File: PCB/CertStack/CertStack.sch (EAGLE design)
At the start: 46 parts, among them J1 MEM2075-00-140-01-A, Q1 SI2302, Q2 SI2302, Q3 SI2302, Q4 SI2302, Q5 MMBT2222A, T1 DMP3098L-7, U1 LT1374CS8-5PBF, U2 INVENSENSE_ICM-20608-GINVENSE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, U3 SST26VF064B-104V/MN

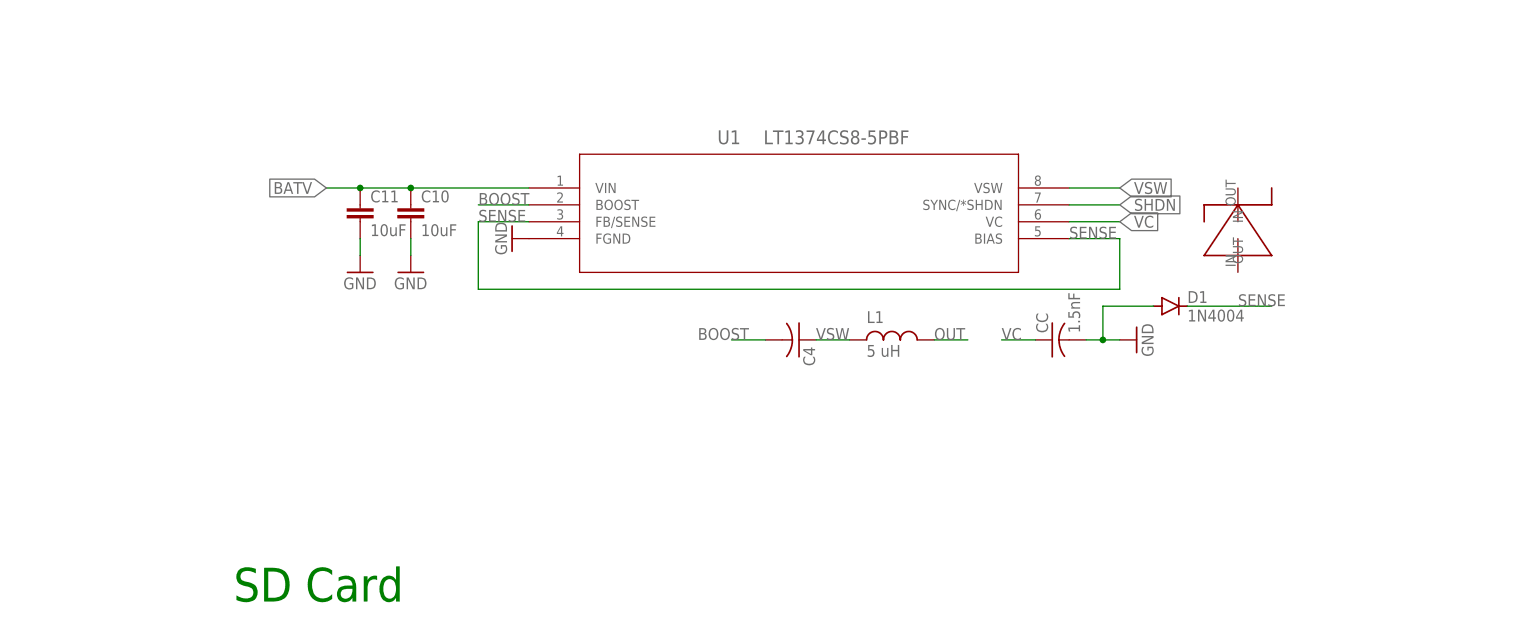
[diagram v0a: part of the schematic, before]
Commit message: PCB
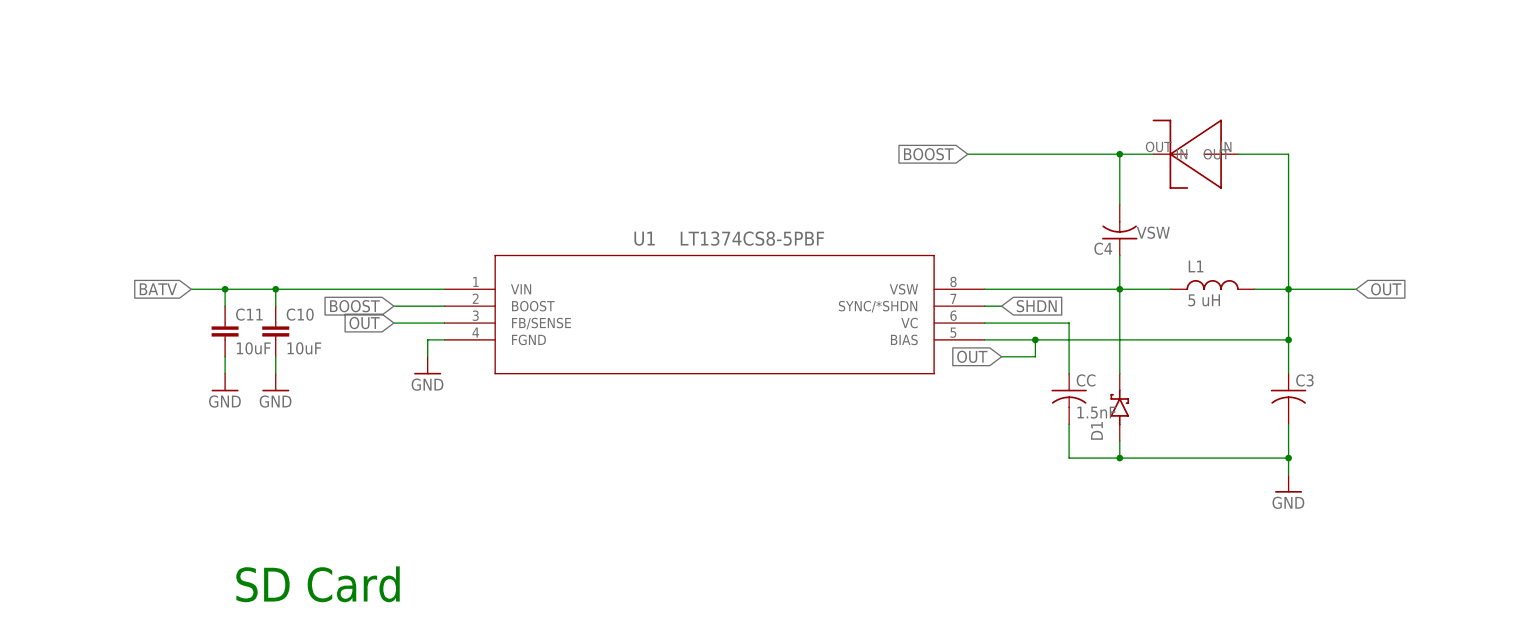
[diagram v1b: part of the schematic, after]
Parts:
- removed U$3: DO-214AB, DO-214AB:DO-214AB
- added C3: (no value), rcl:C-USC0805
- added D2: DO-214AB, DO-214AB:DO-214AB
- D1: value 1N4004 -> PMEG4020ETP,115; device diode:1N4004 -> PMEG4020ETP_115:PMEG4020ETP,115
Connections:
- removed net SENSE: D1.C, U1.BIAS, U1.FB/SENSE
- net BOOST: now also D2.OUT
- net GND: now also C3.2
- net OUT: now also C3.1, D2.IN, U1.BIAS, U1.FB/SENSE
- net VSW: now also D1.K
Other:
- moved on the sheet: C10, C11, C4, CC, L1, U1
